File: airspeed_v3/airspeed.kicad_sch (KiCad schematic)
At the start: 27 parts, among them J1 Header, J2 GPS connector, J3 GPS Header, U1 XGZP6897D, U2 XGZP6897D, U3 BME280, U6 BME280

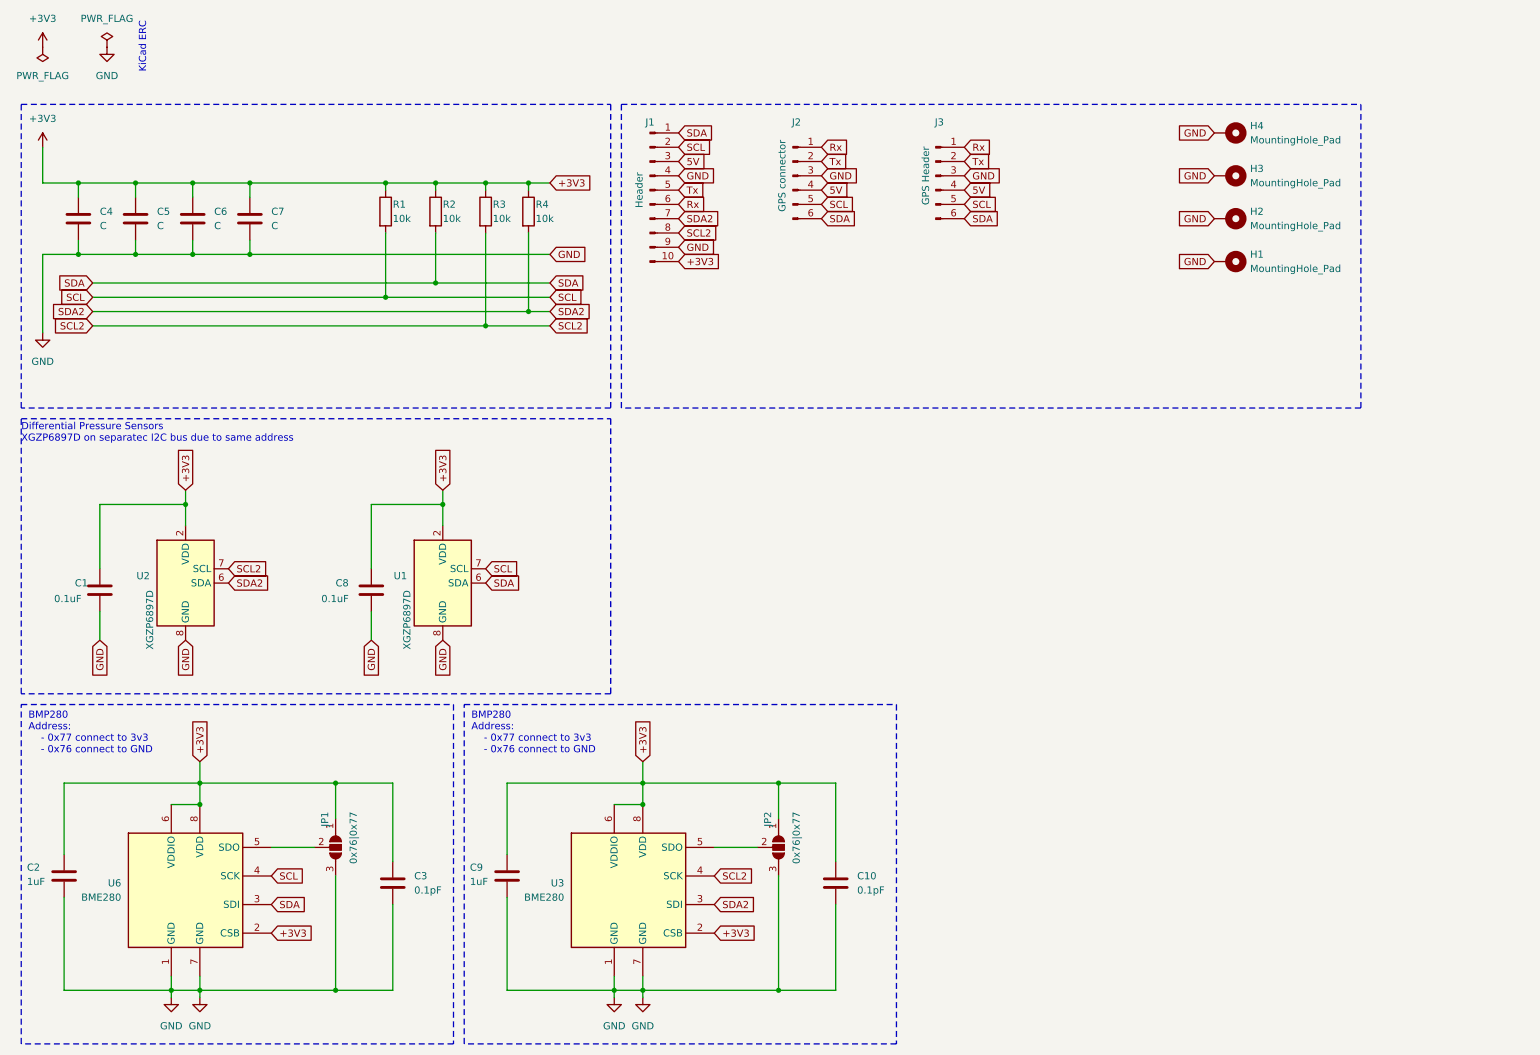
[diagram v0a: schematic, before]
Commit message: airspeed v3.6
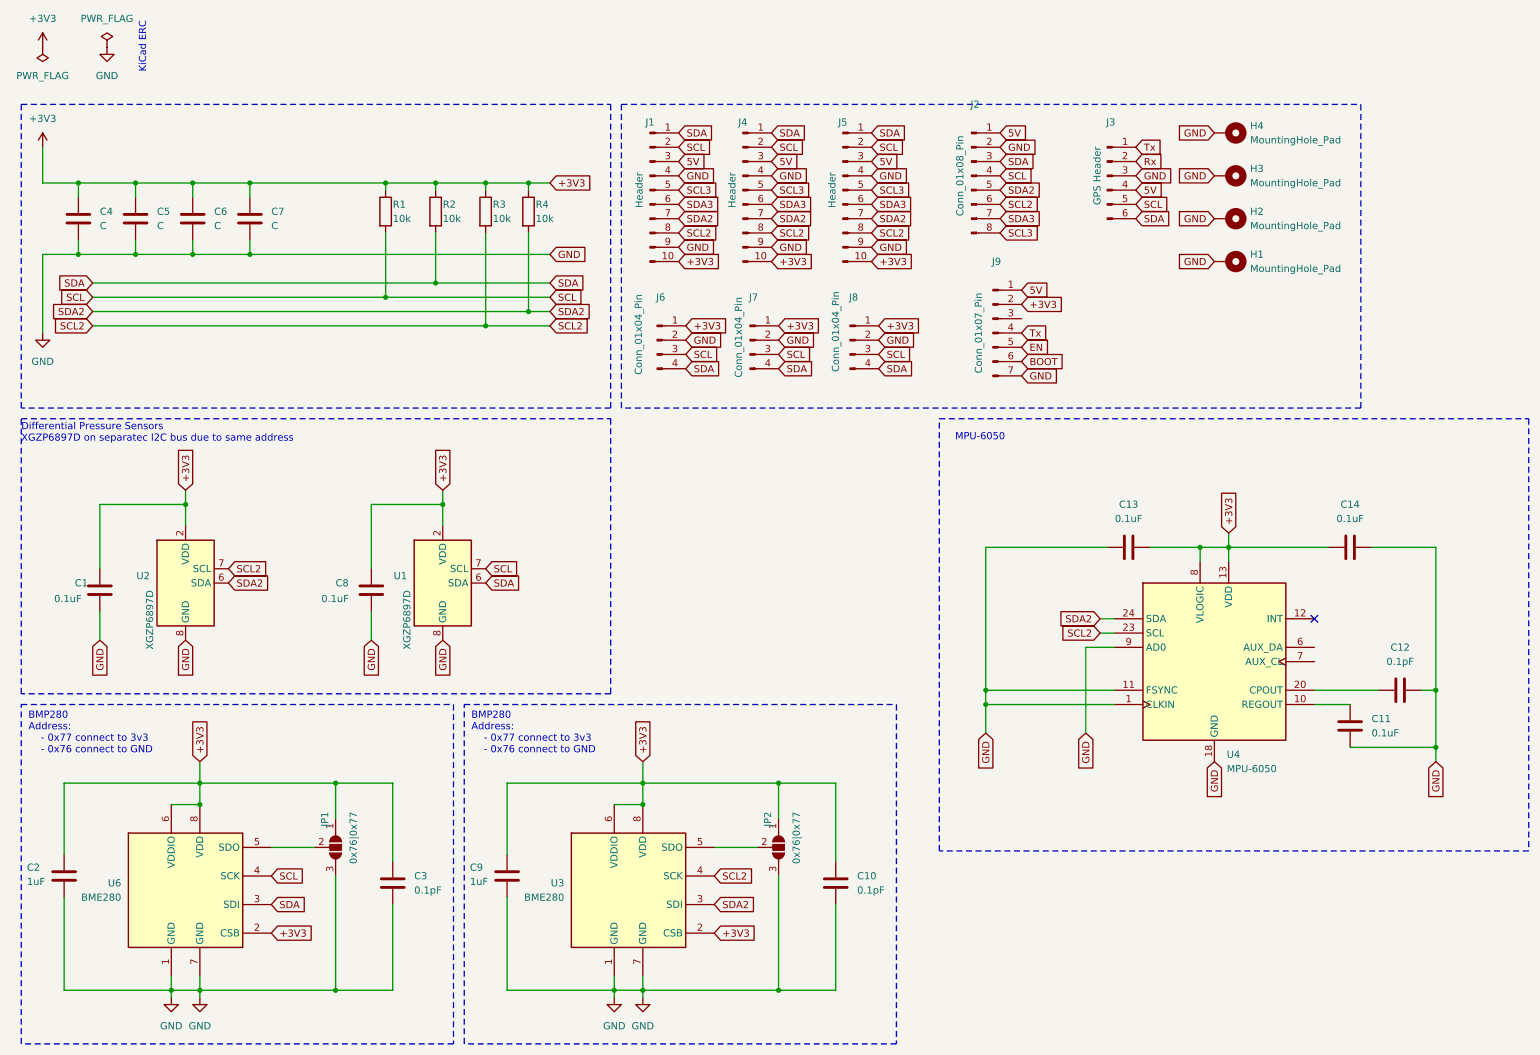
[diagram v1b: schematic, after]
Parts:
- removed J2: GPS connector, Connector_JST:JST_SH_SM06B-SRSS-TB_1x06-1MP_P1.00mm_Horizontal, symbol Connector:Conn_01x06_Pin
- added C11, C13, C14: 0.1uF, Capacitor_SMD:C_0805_2012Metric, symbol Device:C
- added C12: 0.1pF, Capacitor_SMD:C_0805_2012Metric, symbol Device:C
- added J2: Conn_01x08_Pin, Connector_Molex:Molex_PicoBlade_53047-0810_1x08_P1.25mm_Vertical, symbol Connector:Conn_01x08_Pin
- added J4: Header, Connector_PinHeader_2.00mm:PinHeader_1x10_P2.00mm_Vertical, symbol Connector:Conn_01x10_Pin
- added J5: Header, Connector_PinHeader_1.27mm:PinHeader_1x10_P1.27mm_Vertical, symbol Connector:Conn_01x10_Pin
- added J6, J7, J8: Conn_01x04_Pin, Connector_PinHeader_1.27mm:PinHeader_1x04_P1.27mm_Vertical, symbol Connector:Conn_01x04_Pin
- added J9: Conn_01x07_Pin, Connector_Molex:Molex_PicoBlade_53047-0710_1x07_P1.25mm_Vertical, symbol Connector:Conn_01x07_Pin
- added U4: MPU-6050, Sensor_Motion:InvenSense_QFN-24_4x4mm_P0.5mm, symbol Sensor_Motion:MPU-6050
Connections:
- net +3V3: now also C13.2, C14.1, J4.10 (Pin_10), J5.10 (Pin_10), J6.1 (Pin_1), J7.1 (Pin_1), J8.1 (Pin_1), J9.2 (Pin_2), U4.13 (VDD), U4.8 (VLOGIC)
- net 5V: now also J2.1 (Pin_1), J4.3 (Pin_3), J5.3 (Pin_3), J9.1 (Pin_1)
- net GND: now also C11.2, C12.2, C13.1, C14.2, J2.2 (Pin_2), J4.4 (Pin_4), J4.9 (Pin_9), J5.4 (Pin_4), J5.9 (Pin_9), J6.2 (Pin_2), J7.2 (Pin_2), J8.2 (Pin_2), J9.7 (Pin_7), U4.1 (CLKIN), U4.11 (FSYNC), U4.18 (GND), U4.9 (AD0)
- net Rx: now also J3.2 (Pin_2); no longer J1.6 (Pin_6), J3.1 (Pin_1)
- net SCL: now also J2.4 (Pin_4), J4.2 (Pin_2), J5.2 (Pin_2), J6.3 (Pin_3), J7.3 (Pin_3), J8.3 (Pin_3)
- net SCL2: now also J2.6 (Pin_6), J4.8 (Pin_8), J5.8 (Pin_8), U4.23 (SCL)
- net SDA: now also J2.3 (Pin_3), J4.1 (Pin_1), J5.1 (Pin_1), J6.4 (Pin_4), J7.4 (Pin_4), J8.4 (Pin_4)
- net SDA2: now also J2.5 (Pin_5), J4.7 (Pin_7), J5.7 (Pin_7), U4.24 (SDA)
- net Tx: now also J3.1 (Pin_1), J9.4 (Pin_4); no longer J1.5 (Pin_5), J3.2 (Pin_2)
- new net: C11.1, U4.10 (REGOUT)
- new net: C12.1, U4.20 (CPOUT)
- new net BOOT: J9.6 (Pin_6)
- new net EN: J9.5 (Pin_5)
- new net SCL3: J1.5 (Pin_5), J2.8 (Pin_8), J4.5 (Pin_5), J5.5 (Pin_5)
- new net SDA3: J1.6 (Pin_6), J2.7 (Pin_7), J4.6 (Pin_6), J5.6 (Pin_6)
- no-connect marks 0 -> 1
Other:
- note added: "MPU-6050"
- moved on the sheet: J3
